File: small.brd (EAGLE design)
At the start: 19 x 30.1 mm, 4 parts, among them U1 SN74LS241N

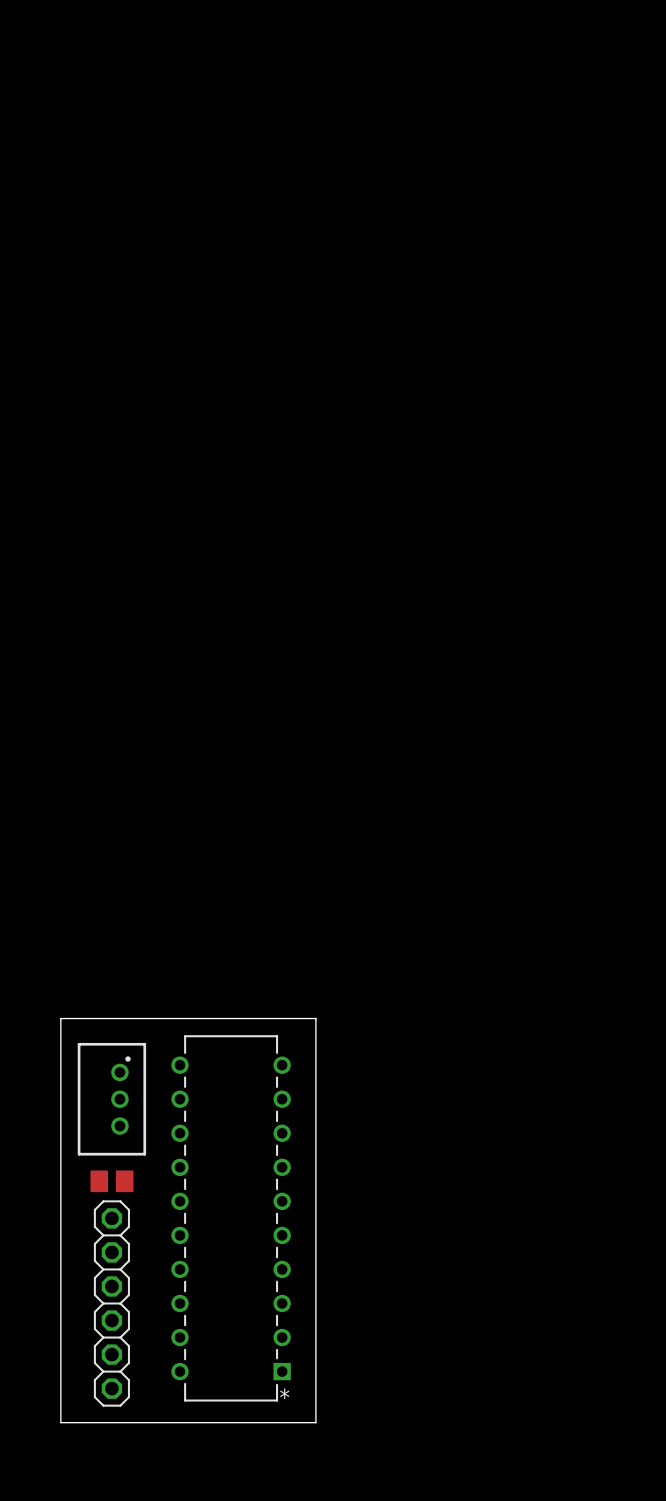
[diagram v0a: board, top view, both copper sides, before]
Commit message: Add files via upload
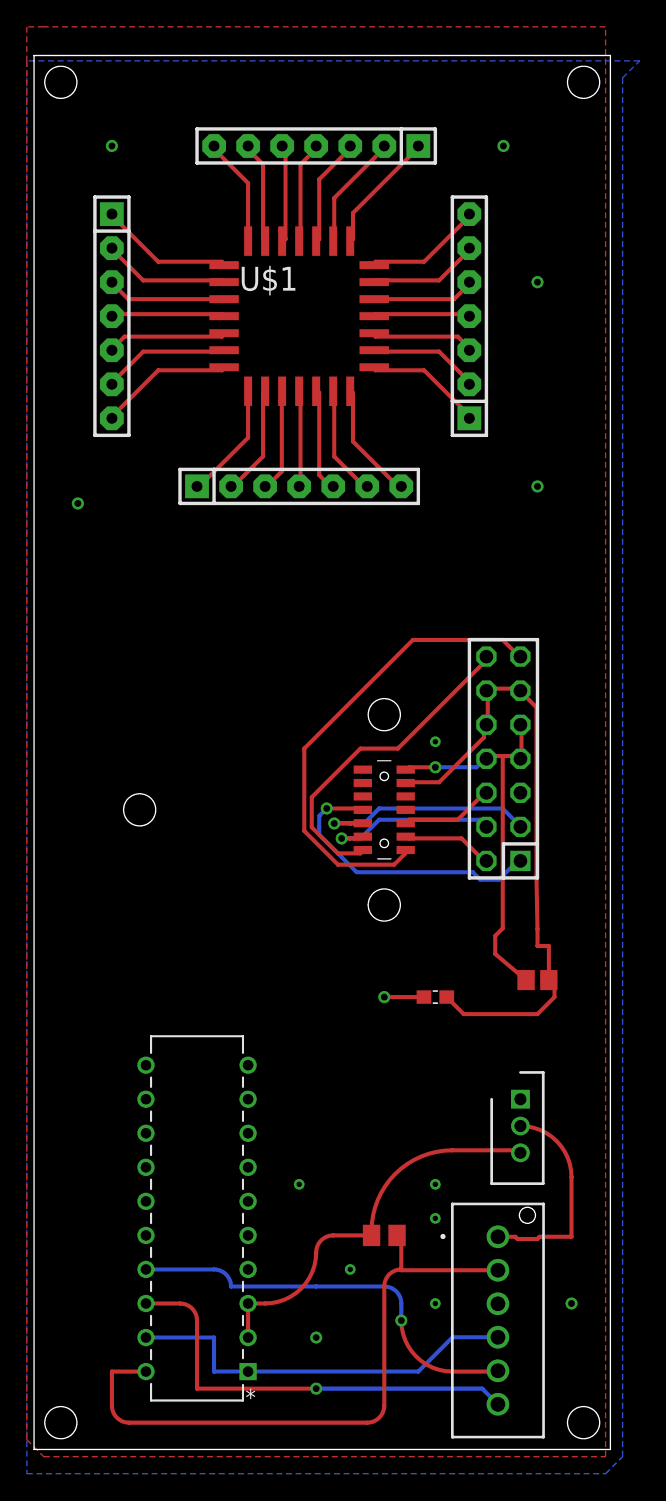
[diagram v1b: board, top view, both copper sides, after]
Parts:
- removed JP1: (no value), adafruit:1X06
- added C8: 10uF, adafruit:C0805
- added C9: 1uF, Common-Parts-Library-Eagle:CC0603KRX7R9BB104_CAPC1608X90
- added J2: 53375-0610, wire to board_molex:53375-0610
- added J3, J4, J5, J6: F-1X07-SIP-100-32, con-headers-jp:SIP-100-07-32
- added J7: CLM-107-02-L-D-A, CLM-107-02-L-D-A:CLM10702LDA
- added J8: F-2X07-DIL-100, con-headers-jp:DIL-100-2X07
- added U$1: IMU, IMU:PLCC28S
- J1: value (none) -> 53253-0370; device Wurth_Connectors_WR-WTB:62000311622 -> xl320_molex:SHDR3W50P0X200_1X3_800X365X570
- moved J1 30.5 mm to (34.3, 24.1), turned to 270 degrees
- moved R1 20.7 mm to (24.1, 14.0)
- moved U1 2.54 mm to (6.35, 26.7)
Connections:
- new net 3.3V: C8.1, C9.1, J7.11, J8.10, J8.11, J8.12
- new net N$1: J4.7, U$1.4
- new net N$10: J3.5, U$1.23
- new net N$11: J3.4, U$1.22
- new net N$12: J3.3, U$1.21
- new net N$13: J3.2, U$1.20
- new net N$14: J3.1, U$1.19
- new net N$15: J6.7, U$1.18
- new net N$16: J6.6, U$1.17
- new net N$17: J6.5, U$1.16
- new net N$18: J6.4, U$1.15
- new net N$19: J6.3, U$1.14
- new net N$2: J4.6, U$1.3
- new net N$20: J6.2, U$1.13
- new net N$21: J6.1, U$1.12
- new net N$22: J5.7, U$1.11
- new net N$23: J5.6, U$1.10
- new net N$24: J5.5, U$1.9
- new net N$25: J5.4, U$1.8
- new net N$26: J5.3, U$1.7
- new net N$27: J5.2, U$1.6
- new net N$28: J5.1, U$1.5
- new net N$3: J4.5, U$1.2
- new net N$4: J4.4, U$1.1
- new net N$5: J4.3, U$1.28
- new net N$59: J7.1, J8.13
- new net N$6: J4.2, U$1.27
- new net N$60: J7.2, J8.14
- new net N$61: J7.3, J8.2
- new net N$62: J7.4, J8.4
- new net N$63: J7.5, J8.6
- new net N$64: J7.8, J8.1
- new net N$65: J7.6, J8.3
- new net N$7: J4.1, U$1.26
- new net N$8: J3.7, U$1.25
- new net N$9: J3.6, U$1.24
- net 5V: now also J2.2; no longer JP1.2
- net 7.4V: now also J2.1; no longer JP1.1
- net DATA_CONTROL: now also J2.4; no longer JP1.4
- net GND: now also C8.2, C9.2, J2.3, J7.13, J8.7, J8.8, J8.9; no longer JP1.3
- net RX: now also J2.6; no longer JP1.6
- net TX: now also J2.5; no longer JP1.5
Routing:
- net 5V: track 0.00 -> 47.3 mm
- net 3.3V: track 0.00 -> 47.0 mm
- net N$59: track 0.00 -> 35.3 mm
- net GND: track 0.00 -> 32.6 mm, vias 0 -> 15
- net RX: track 0.00 -> 32.4 mm, vias 0 -> 1
- net TX: track 0.00 -> 30.2 mm, vias 0 -> 1
- net DATA_CONTROL: track 0.00 -> 29.9 mm
- net DATA: track 0.00 -> 27.9 mm
- net N$60: track 0.00 -> 24.6 mm
- net N$64: track 0.00 -> 21.9 mm, vias 0 -> 1
- net N$65: track 0.00 -> 17.1 mm, vias 0 -> 1
- net 7.4V: track 0.00 -> 15.5 mm
- net N$62: track 0.00 -> 13.2 mm, vias 0 -> 1
- net N$22: track 0.00 -> 10.0 mm
- net N$28: track 0.00 -> 10.0 mm
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- added copper zone on layer 1, net GND
- added copper zone on layer 16, net GND
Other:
- board size 19 x 30.1 mm -> 43 x 104 mm
